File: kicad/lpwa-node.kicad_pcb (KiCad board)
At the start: 4 copper layers, 85 x 55 mm, 86 parts, among them J1 USB_C_ESP, J4 USB_C_SIM, J5 SIM_Card, J6 MEAS, J8 LTE, SW1 BOOT, SW2 USER, U1 TPS7A0230PDBVR, U10 LM66100DCK, U11 LM66100DCK, U2 USBLC6-2SC6, U3 ESP32-C3-WROOM-02, U4 AHT20, U5 BH-AA-B6AA044, U6 SIM7080G, U7 TXU0204PWR, U8 USBLC6-2SC6, U9 TLV75901PDRVR

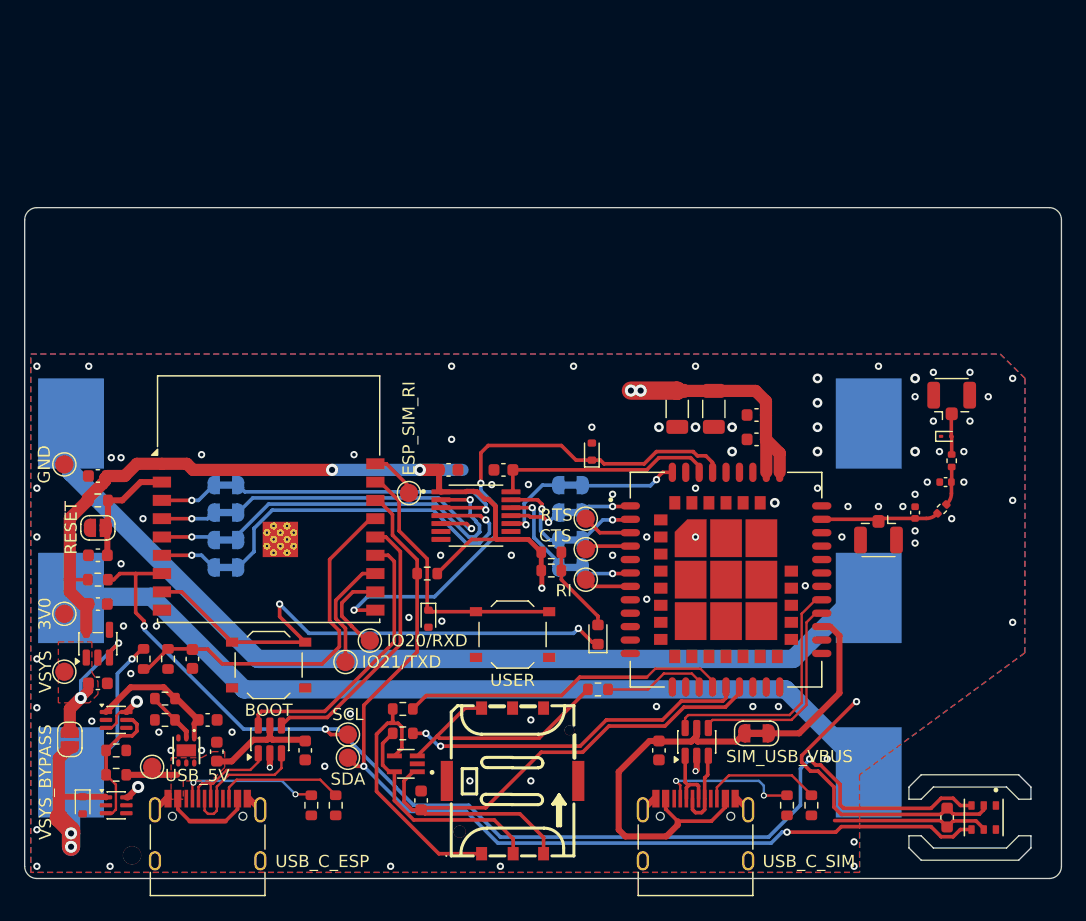
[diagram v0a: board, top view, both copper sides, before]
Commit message: Draft
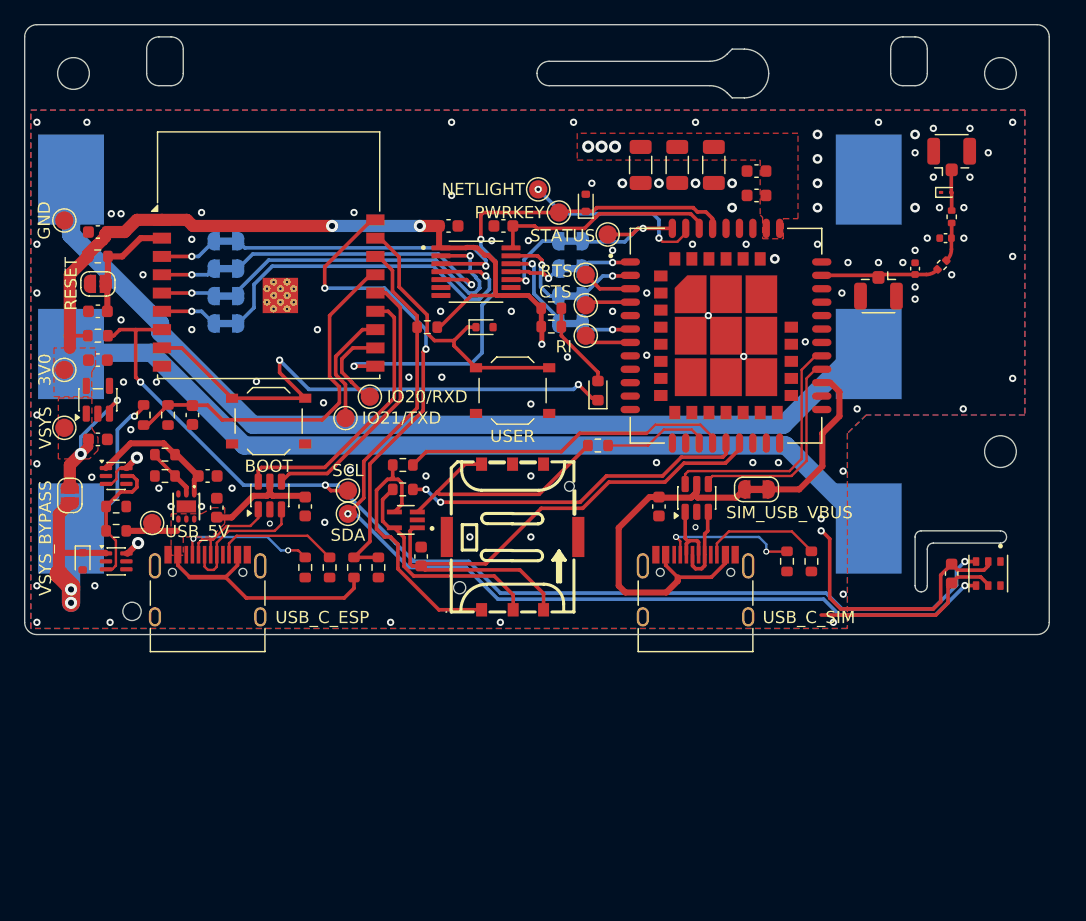
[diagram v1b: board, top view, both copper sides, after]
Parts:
- removed TP3: ESP_SIM_RI, TestPoint:TestPoint_Pad_D1.5mm
- added C22: 100µF, Capacitor_SMD:C_1206_3216Metric, F.Cu at (100.5, 46.5)
- added R23: 1M, Resistor_SMD:R_0603_1608Metric, F.Cu at (79.0, 79.5)
- added R24: 732k, Resistor_SMD:R_0603_1608Metric, F.Cu at (77.0, 79.5)
- added TP13: PWRKEY, TestPoint:TestPoint_Pad_D1.5mm, F.Cu at (93.8, 50.4)
- added TP14: STATUS, TestPoint:TestPoint_Pad_D1.5mm, F.Cu at (97.8, 52.2)
- added TP15: NETLIGHT, TestPoint:TestPoint_Pad_D1.5mm, F.Cu at (92.1, 48.5)
- moved D2 24.3 mm to (87.7, 59.8), turned to 0 degrees
- moved D4 20.4 mm to (96.0, 49.6)
- moved R1 20.2 mm to (83.0, 59.8)
- moved U4 20.0 mm to (129.0, 80.0)
- moved C6 20.0 mm to (126.0, 80.0)
- moved C1 20.0 mm to (56.0, 69.0)
- moved C10 20.0 mm to (110.0, 47.0)
- moved C11 20.0 mm to (106.5, 46.5)
- moved C12 20.0 mm to (89.2, 51.5)
- moved C13 20.0 mm to (103.5, 46.5)
- moved C14 20.0 mm to (82.5, 78.6)
- moved C15 20.0 mm to (102.0, 74.5)
- moved C17 20.0 mm to (123.0, 55.0)
- moved C19 20.0 mm to (125.5, 52.5)
- moved C2 20.0 mm to (56.0, 58.5)
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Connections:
- U3 pad 18: ESP_SIM_RI -> ESP_USB_SENSE
- U6 pad 41: unconnected-(U6-NETLIGHT-Pad41) -> Net-(U6-NETLIGHT)
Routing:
- net ESP_USB_SENSE: track 0.00 -> 40.3 mm, vias 0 -> 2
- net VSYS: track 106.0 -> 83.1 mm, vias 6 -> 7
- net Net-(U6-NETLIGHT): track 0.00 -> 15.5 mm, vias 0 -> 2
- net USB_ESP_+5V: track 20.8 -> 33.2 mm
- net 3V0: track 126.7 -> 117.8 mm
- net GND: track 21.2 -> 16.1 mm, vias 90 -> 105
- net SCL: track 94.1 -> 89.7 mm
- net ESP_SIM_RI: track 4.07 -> 0.00 mm
- net SIM_STATUS: track 7.88 -> 11.0 mm
- net Net-(U5-Pad2): track 77.8 -> 79.2 mm
- net ESP_BTN: track 22.5 -> 23.5 mm
- net SIM_PWRKEY: track 44.6 -> 45.4 mm
- net SDA: track 80.3 -> 81.0 mm
- added copper zone on F.Cu, net 3V0
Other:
- board size 85 x 55 mm -> 84 x 50 mm
- board text added: "ENGINEERING SAMPLE NOT FOR RESALE NOT CERTIFIED"
- board text added: "https://github.com/MikkoTervala/ lpwa-node-hardware"
- board text added: "⌀ 2.6mm"
- board text removed: "NiMH Rechargeable = Best Alkaline = OK Lithium 1.5V = NOT ALLOWED!"
